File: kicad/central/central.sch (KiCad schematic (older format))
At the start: 4 parts

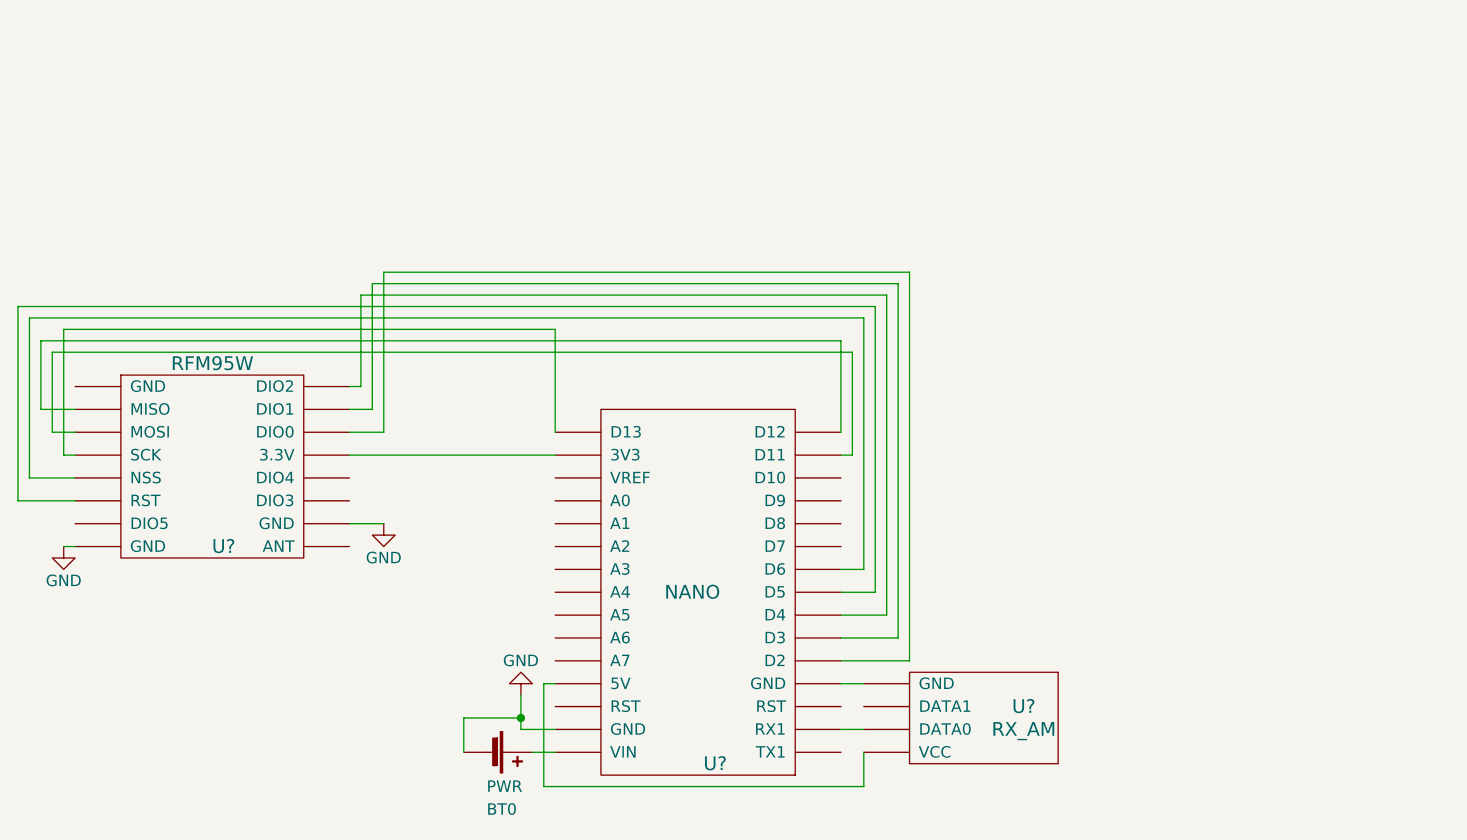
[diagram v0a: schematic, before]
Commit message: Esquemático da central atualizado
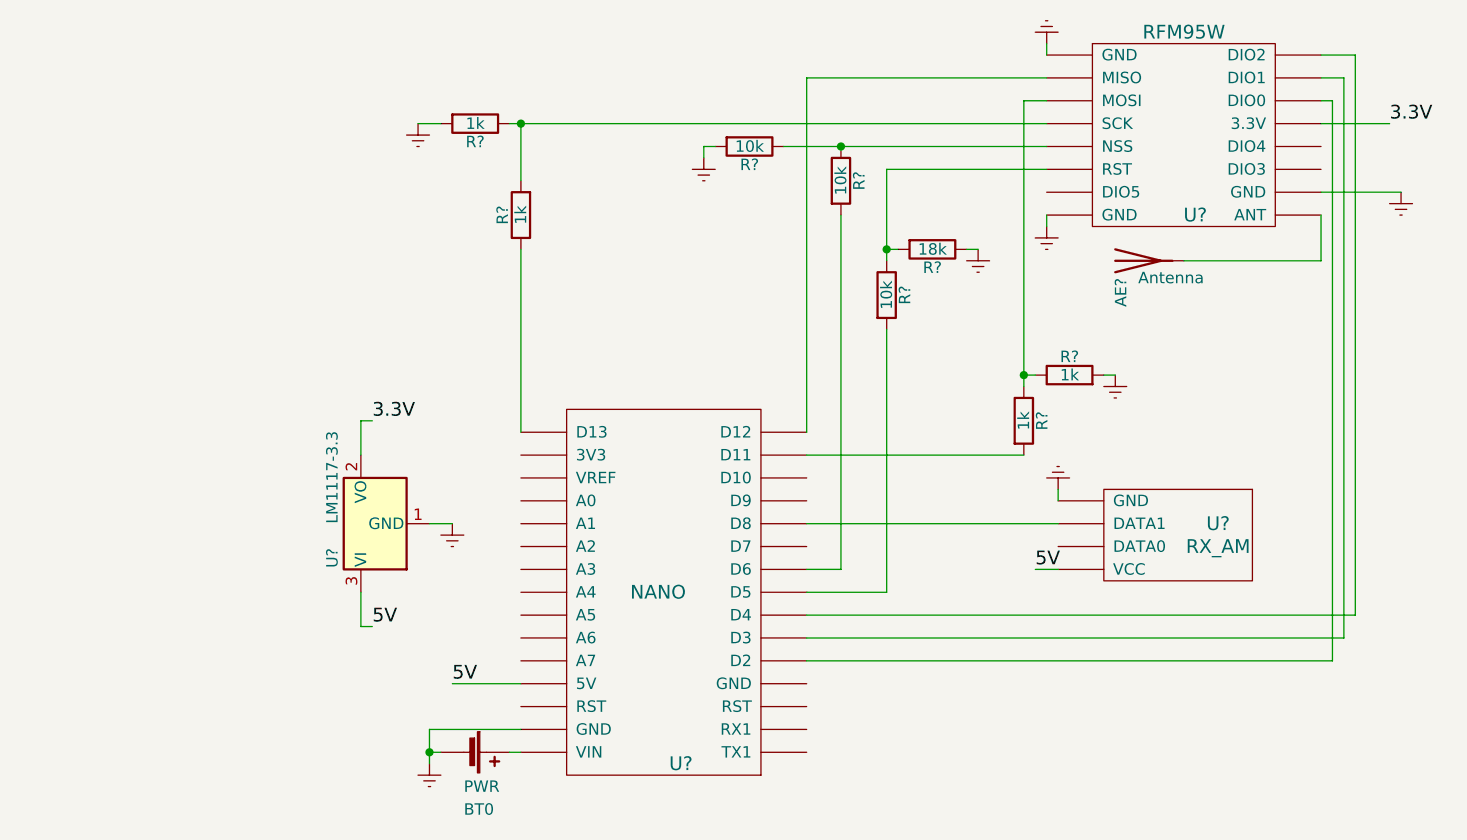
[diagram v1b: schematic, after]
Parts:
- added AE?: Antenna, symbol Antenna
- added R? (x3): 10k, symbol R
- added R? (x4): 1k, symbol R
- added R?: 18k, symbol R
- added U?: LM1117-3.3, symbol LM1117-3.3
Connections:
- net GND is gone; now on net Earth: BT0.2 (-), U?.~ (SCK), U?.~ (VREF)
- net Earth: now reaches U?.~ (VREF)
- net Earth: now also U?.~ (VCC), R?.1, R?.2, R?.2, R?.2, U?.1 (GND)
- new net: U?.~ (VCC), U?.~ (VREF)
- new net: U?.~ (SCK), U?.~ (VREF) (x4)
- new net: R?.2, U?.~ (VREF) (x3)
- new net: R?.1, U?.~ (VREF)
- new net: AE?.1 (A), U?.~ (SCK)
- new net: R?.1, R?.2, U?.~ (SCK) (x2)
- new net: R?.1, R?.1, U?.~ (SCK) (x2)
- new net 3.3V: U?.2 (VO), U?.~ (SCK)
- new net 5V: U?.3 (VI), U?.~ (VCC), U?.~ (VREF)
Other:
- moved on the sheet: BT0, U?
